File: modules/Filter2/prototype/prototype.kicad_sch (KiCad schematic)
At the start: 31 parts, among them J1 Conn_01x09, U1 TL072, U2 TL074

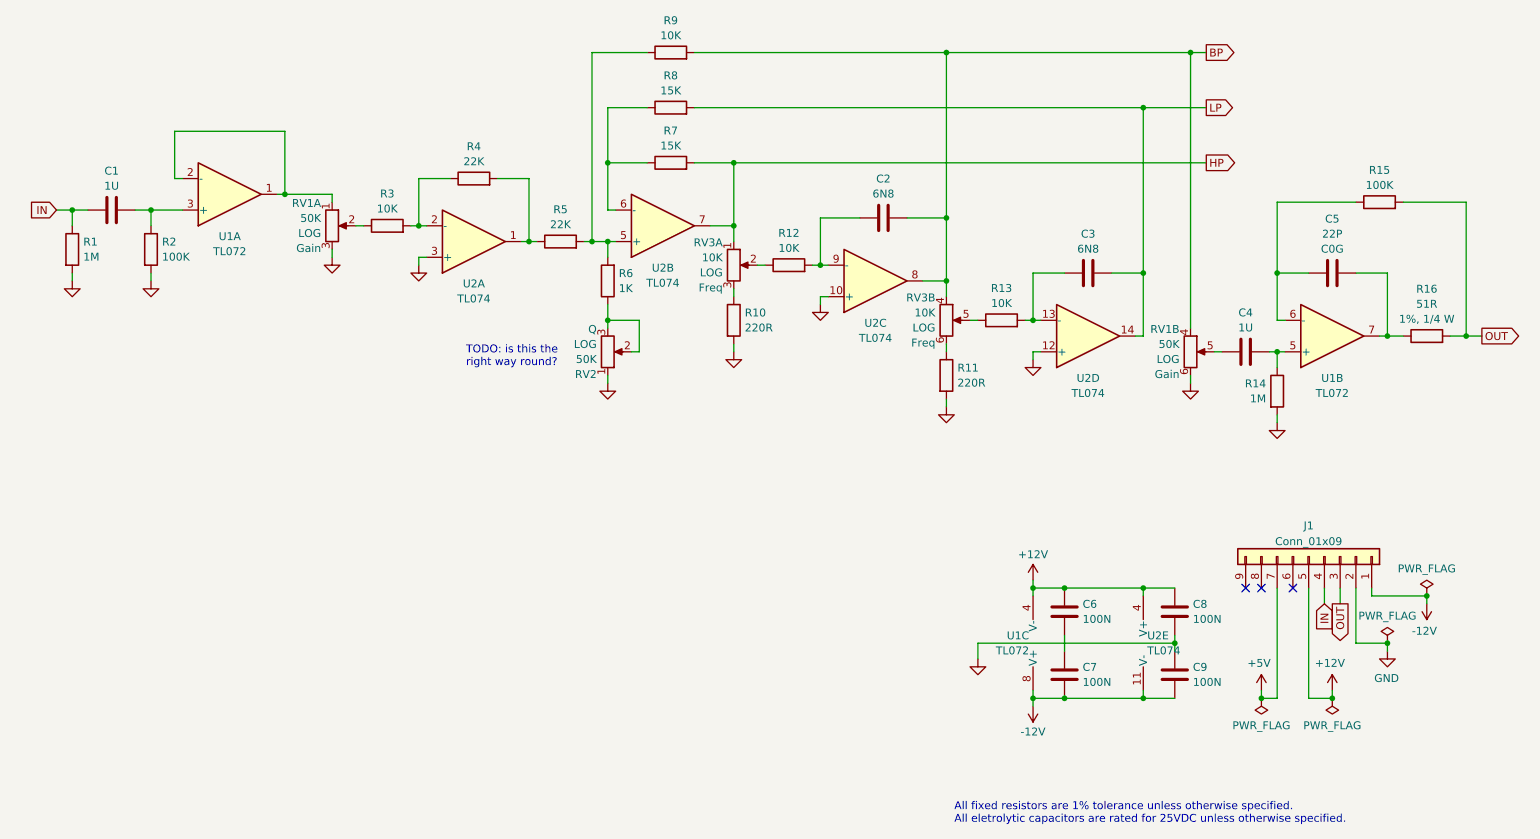
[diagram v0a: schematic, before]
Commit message: Filter2 prototype - wip
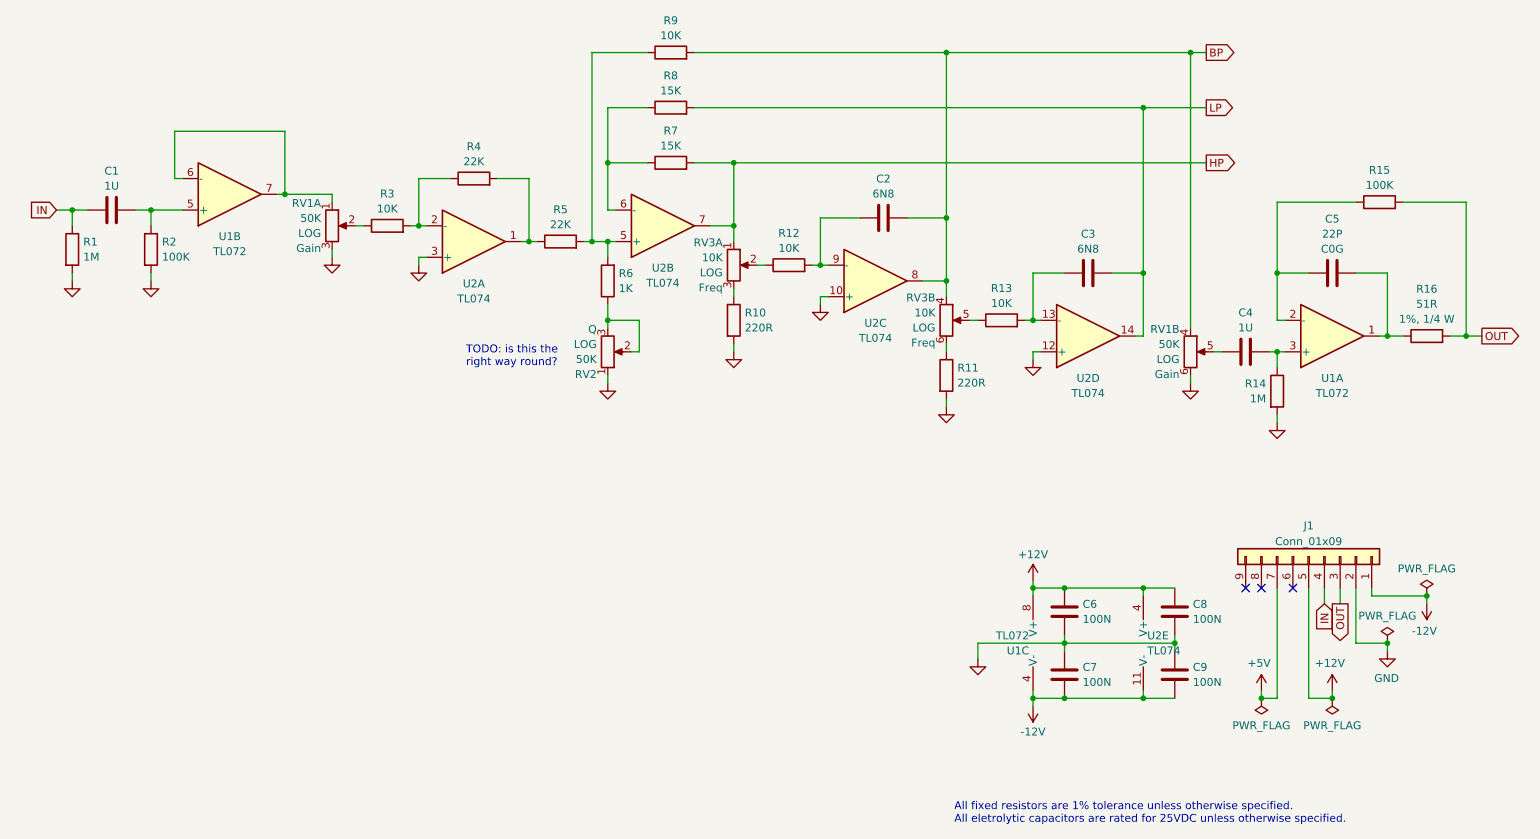
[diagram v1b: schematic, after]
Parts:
- C1, C2, C3, C4: footprint (none) -> -lmp-misc:C_Rect_Kemet_L7.2mm_W2.5mm_P5mm
- C5: footprint (none) -> -lmp-misc:C_Disc_D5.0mm_W2.5mm_P2.50mm
- R1, R14, R2, R4, R7: footprint -lmp-misc:R_Axial_DIN0207_L6.3mm_D2.5mm_P7.62mm_Horizontal -> -lmp-stripboard:SB_Gen_1
- R16: footprint -lmp-misc:R_Axial_DIN0207_L6.3mm_D2.5mm_P10.16mm_Horizontal -> -lmp-stripboard:SB_Gen_2
- R5: footprint -lmp-misc:R_Axial_DIN0207_L6.3mm_D2.5mm_P7.62mm_Horizontal -> -lmp-stripboard:SB_Gen_4
- R6: footprint -lmp-misc:R_Axial_DIN0207_L6.3mm_D2.5mm_P7.62mm_Horizontal -> -lmp-stripboard:SB_Gen_7
- RV1, RV3: footprint (none) -> -lmp-synth:Potentiometer_Alpha_RD902F-40-00D_Dual_Vertical
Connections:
- net +12V: now also U1.8 (V+); no longer U1.4 (V-)
- net -12V: now also U1.4 (V-); no longer U1.8 (V+)
- net GND: now also C6.2, C7.1
- net at C1.2, R2.1: now also U1.5 (+); no longer U1.3 (+)
- net at C4.2, R14.1: now also U1.3 (+); no longer U1.5 (+)
- net at C5.1, R15.1: now also U1.2 (-); no longer U1.6 (-)
- net at C5.2, R16.1: now also U1.1; no longer U1.7
- new net: RV1.1, U1.6 (-), U1.7

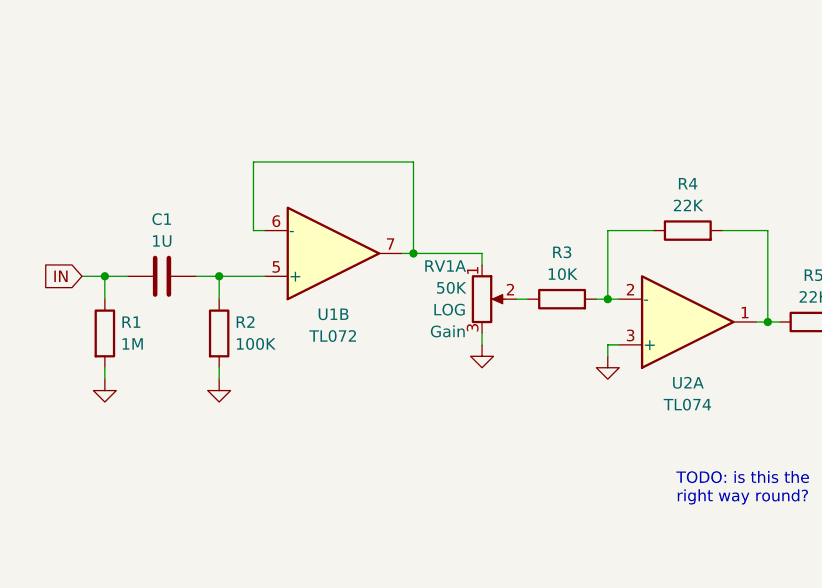
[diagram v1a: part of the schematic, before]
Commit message: Filter2 prototype
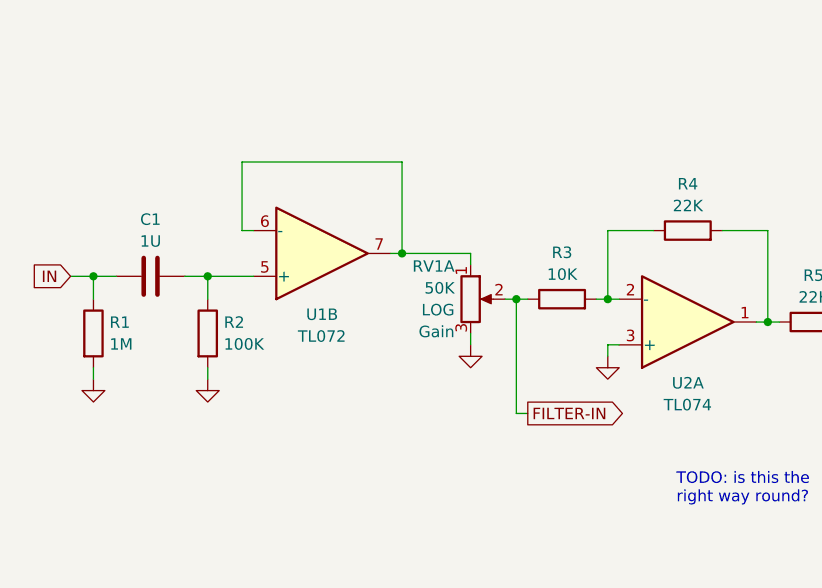
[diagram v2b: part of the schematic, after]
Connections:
- net FILTER-IN: now reaches R3.1, RV1.2
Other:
- moved on the sheet: C1, R1, R2, RV1A, U1B
